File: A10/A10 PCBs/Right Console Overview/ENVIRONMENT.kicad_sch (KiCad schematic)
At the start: 20 parts, among them J20 Conn_01x02_Female, J21 ENVIRONMENT, SW15 EMEGY NORM TEST, SW16 NORM / RAM, SW17 POTIT HEAT, SW18 100% OXY, SW19 OXY IND TEST, SW20 MAIN AIR, SW21 NVG, SW22 BLEED AIR

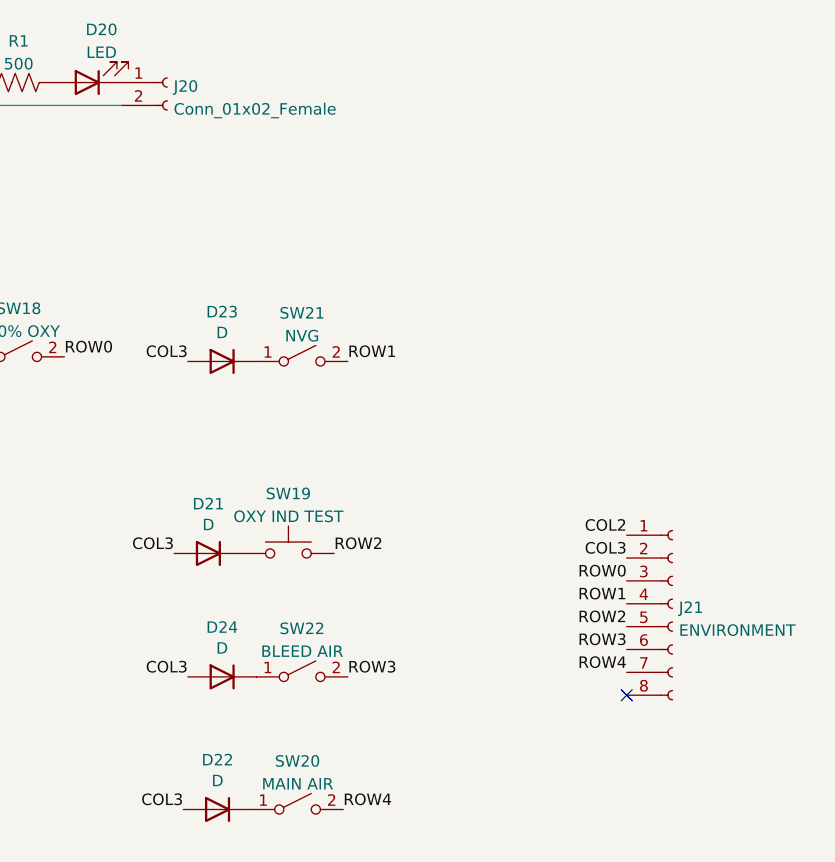
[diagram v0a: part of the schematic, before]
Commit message: a10
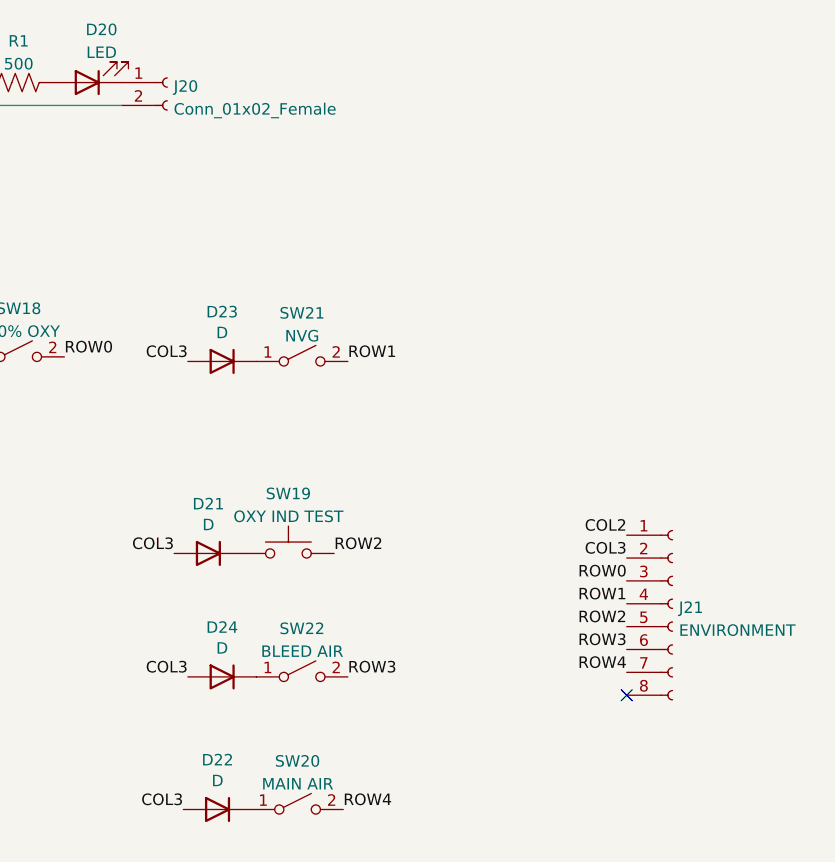
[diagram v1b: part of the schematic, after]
